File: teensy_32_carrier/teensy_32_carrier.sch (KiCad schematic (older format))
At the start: 27 parts, among them J1 CON_01X03_PTH_2.54MM, J10 CJ, J11 CJ, J12 CJ, J13 CJ, J2 CON_01X08_PTH_2.54MM, J3 CON_01X06_PTH_2.54MM, J4 CON_01X04_PTH_2.54MM, J5 CON_01X03_PTH_2.54MM, J6 CON_01X03_PTH_2.54MM, J7 CON_01X08_PTH_2.54MM, J8 CON_01X05_PTH_2.54MM, P1 S9200-ND, SW1 TACT_6MM, SW2 TACT_6MM, U1 ED3052-5-ND, U2 SAM10855-ND

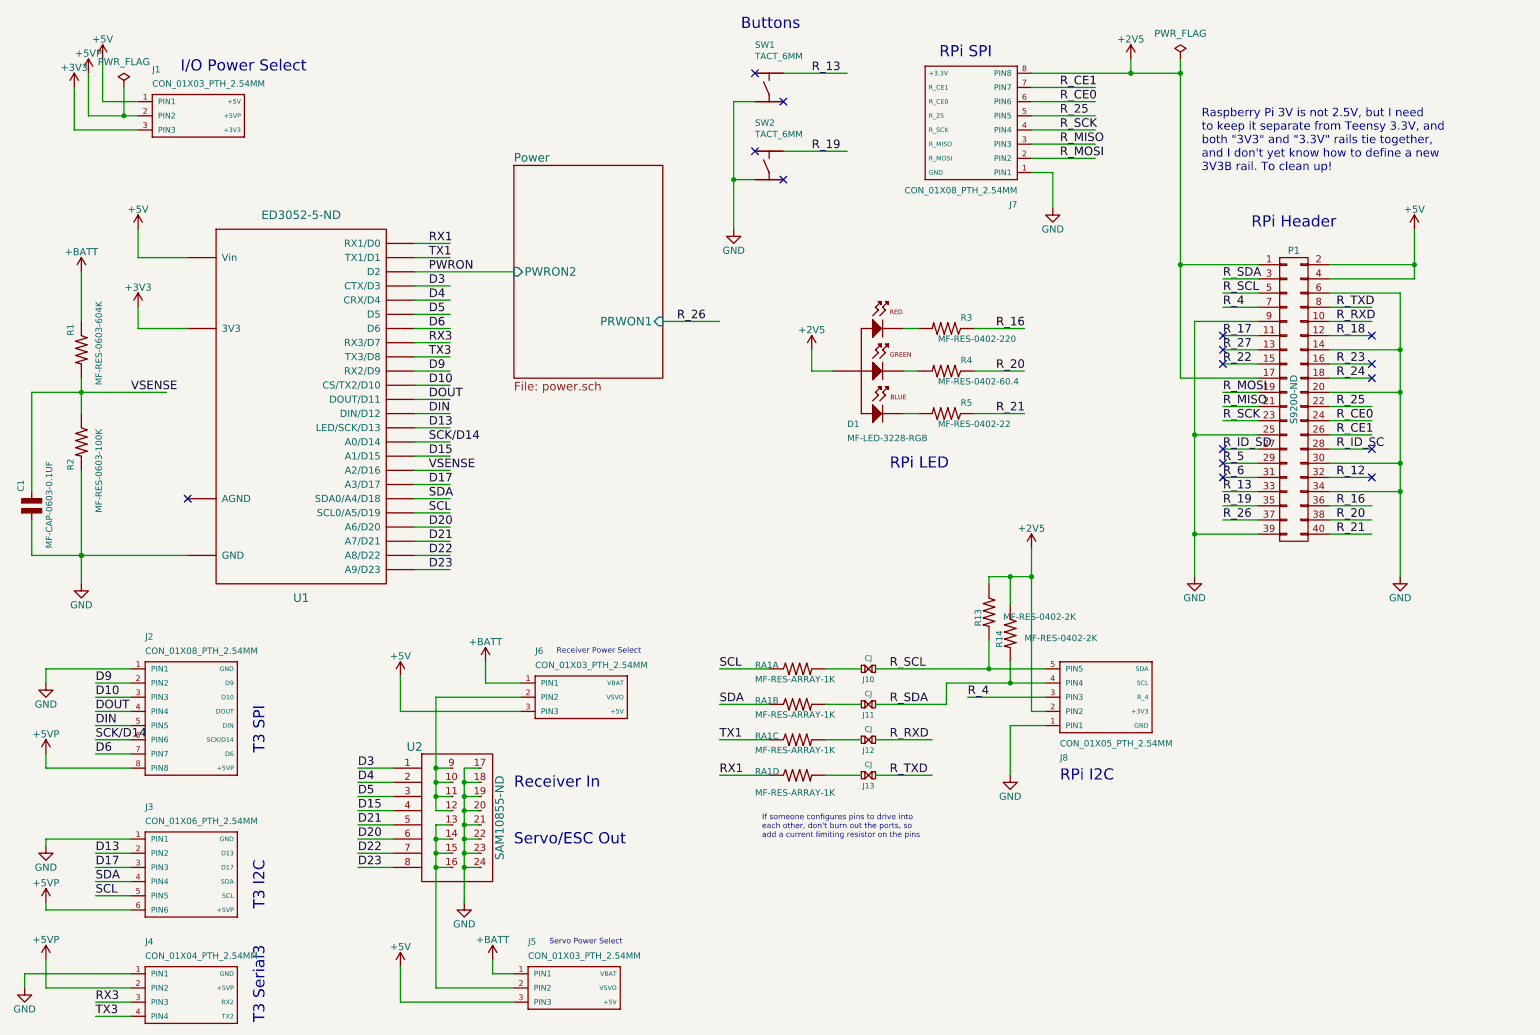
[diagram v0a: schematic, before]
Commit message: Choose a part for screw terminals.
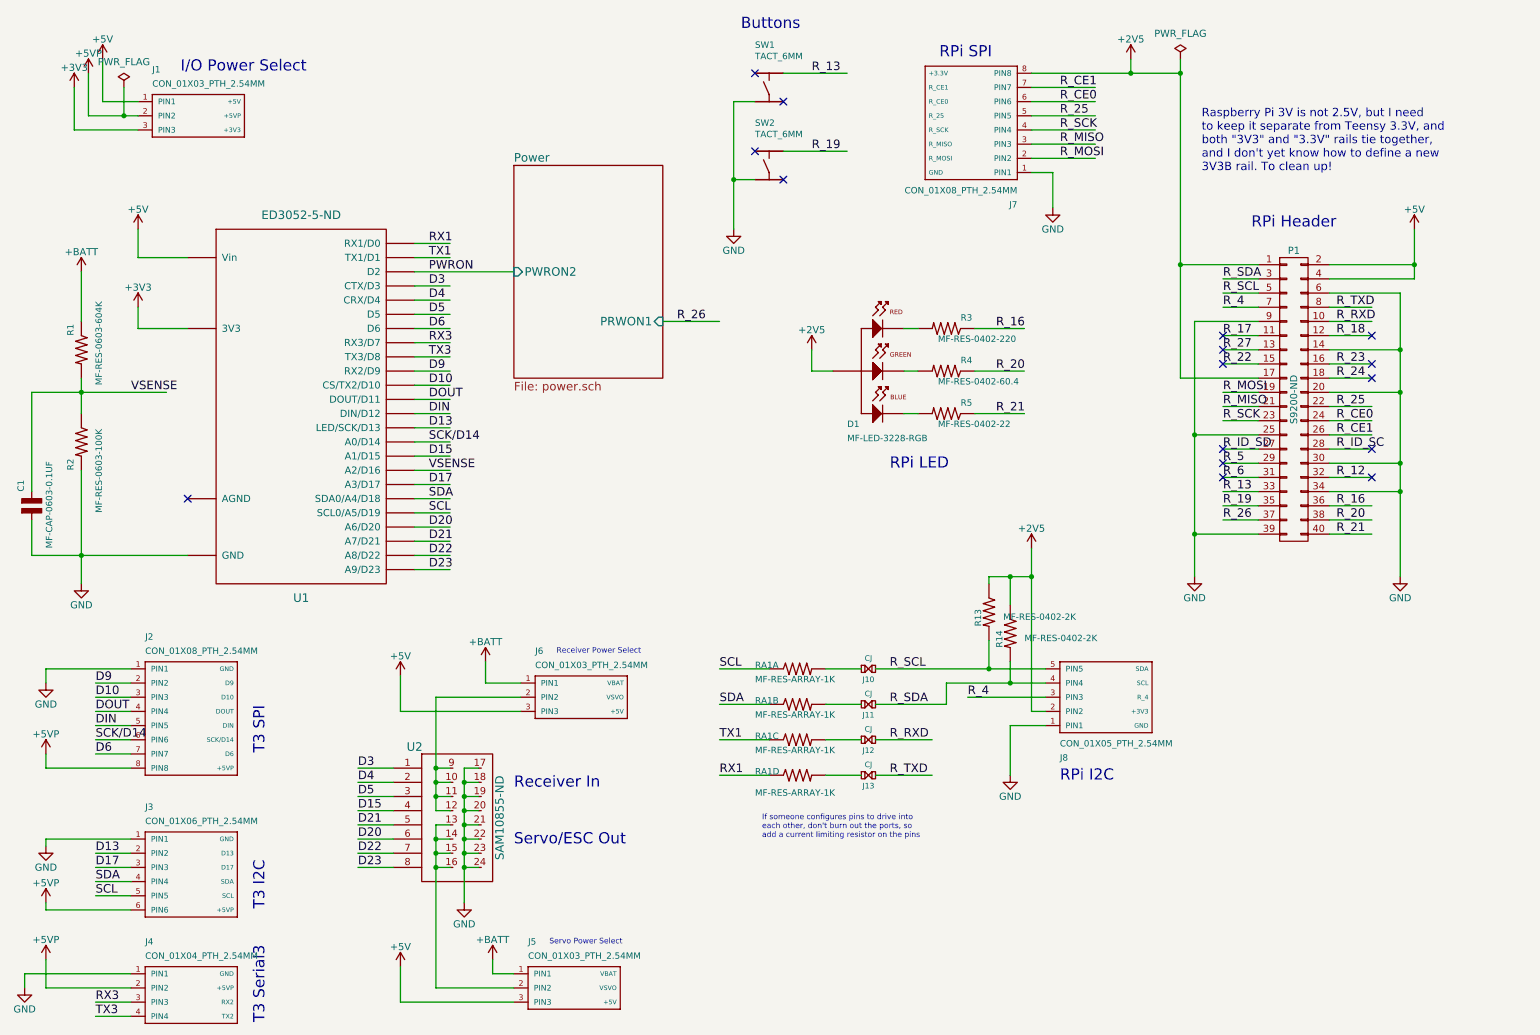
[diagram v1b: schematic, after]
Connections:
- wire segments 229 -> 195
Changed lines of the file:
@@
 	3850 5850 3750 5850
 Wire Wire Line
-	3750 5850 3750 5950
-Wire Wire Line
-	3750 5950 3750 6050
-Wire Wire Line
-	3750 6050 3750 6150
-Wire Wire Line
-	3750 6150 3750 6250
-Wire Wire Line
-	3750 6250 3750 6350
-Wire Wire Line
-	3750 6350 3750 6450
-Wire Wire Line
-	3750 6450 3750 6550
-Wire Wire Line
-	3750 6550 3750 6800
+	3750 5850 3750 6800
 Wire Wire Line
 	3850 6550 3750 6550
@@
 	3650 5850 3550 5850
 Wire Wire Line
-	3550 5350 3550 5850
-Wire Wire Line
-	3550 5850 3550 5950
-Wire Wire Line
-	3550 5950 3550 6050
-Wire Wire Line
-	3550 6050 3550 6150
+	3550 5350 3550 6150
 Wire Wire Line
 	3550 5950 3650 5950
@@
 	3650 6250 3550 6250
 Wire Wire Line
-	3550 6250 3550 6350
-Wire Wire Line
-	3550 6350 3550 6450
-Wire Wire Line
-	3550 6450 3550 6550
-Wire Wire Line
-	3550 6550 3550 7400
+	3550 6250 3550 7400
 Wire Wire Line
 	3650 6350 3550 6350
@@
 $EndComp
 Wire Wire Line
-	1100 1250 1350 1250
-Wire Wire Line
-	1350 1250 1450 1250
+	1100 1250 1450 1250
 Wire Wire Line
 	1100 1250 1100 950
@@
 TX3
 Wire Wire Line
-	1050 3750 1050 4350
-Wire Wire Line
-	1050 4350 1050 4350
+	1050 3750 1050 4550
 $Comp
 L RESISTOR_0402 R2
@@
 $EndComp
 Wire Wire Line
-	1050 3100 1050 3200
-Wire Wire Line
-	1050 3200 1050 3350
+	1050 3100 1050 3350
 $Comp
 L RESISTOR_0402 R1
@@
 Connection ~ 1050 4350
 Wire Wire Line
-	700  3200 1050 3200
-Wire Wire Line
-	1050 3200 1650 3200
+	700  3200 1650 3200
 Wire Wire Line
 	700  3200 700  3900
@@
 	8800 2300 9350 2300
 Wire Wire Line
-	8800 850  8800 950
-Wire Wire Line
-	8800 950  8800 2300
-Wire Wire Line
-	8800 2300 8800 3100
+	8800 850  8800 3100
 Wire Wire Line
 	9100 2400 9350 2400
@@
 	9100 2600 9350 2600
 Wire Wire Line
-	8900 2700 8900 3500
-Wire Wire Line
-	8900 3500 8900 4200
-Wire Wire Line
-	8900 4200 8900 4500
+	8900 2700 8900 4500
 Wire Wire Line
 	8900 2700 9350 2700
@@
 Connection ~ 8900 4200
 Wire Wire Line
-	10450 2050 10450 2300
-Wire Wire Line
-	10450 2300 10450 2400
+	10450 2050 10450 2400
 Wire Wire Line
 	10450 2300 9850 2300
@@
 	9850 2500 10350 2500
 Wire Wire Line
-	10350 2500 10350 2900
-Wire Wire Line
-	10350 2900 10350 3200
-Wire Wire Line
-	10350 3200 10350 3700
-Wire Wire Line
-	10350 3700 10350 3900
-Wire Wire Line
-	10350 3900 10350 4500
+	10350 2500 10350 4500
 $Comp
 L GND #PWR018
@@
 	1    0    0    -1
 $EndComp
-Wire Wire Line
-	1050 4350 1050 4550
 $Comp
 L GND #PWR021
@@
 $EndComp
 Wire Wire Line
-	7750 950  8450 950
-Wire Wire Line
-	8450 950  8800 950
+	7750 950  8800 950
 Connection ~ 8450 950
 Wire Wire Line
@@
 	5800 1150 5650 1150
 Wire Wire Line
-	5650 1150 5650 1700
-Wire Wire Line
-	5650 1700 5650 2050
+	5650 1150 5650 2050
 Wire Wire Line
 	5800 1700 5650 1700
@@
 R_SDA
 Wire Wire Line
-	7750 4300 7750 4500
-Wire Wire Line
-	7750 4500 7750 5450
-Wire Wire Line
-	6650 5150 7450 5150
-Wire Wire Line
-	7450 5150 7850 5150
-Wire Wire Line
-	7150 5250 7600 5250
-Wire Wire Line
-	7600 5250 7850 5250
+	7750 4300 7750 5450
+Wire Wire Line
+	6650 5150 7850 5150
+Wire Wire Line
+	7150 5250 7850 5250
 $Comp
 L RESISTOR_0402 R13
@@
 $EndComp
 Wire Wire Line
-	7450 4500 7600 4500
-Wire Wire Line
-	7600 4500 7750 4500
+	7450 4500 7750 4500
 Connection ~ 8800 950
 Wire Wire Line
 	8450 950  8450 850
 Wire Wire Line
-	1800 4350 1050 4350
+	700  4350 1800 4350
 NoConn ~ 1800 3950
 Wire Wire Line
 	700  4350 700  4100
-Wire Wire Line
-	700  4350 1050 4350
-Connection ~ 1050 4350
 $EndSCHEMATC
